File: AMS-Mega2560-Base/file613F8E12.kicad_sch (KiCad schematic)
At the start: 8 parts, among them IC18 MAX31865AAP+, J28 Conn_01x02, J29 Conn_01x03, J30 Conn_01x02

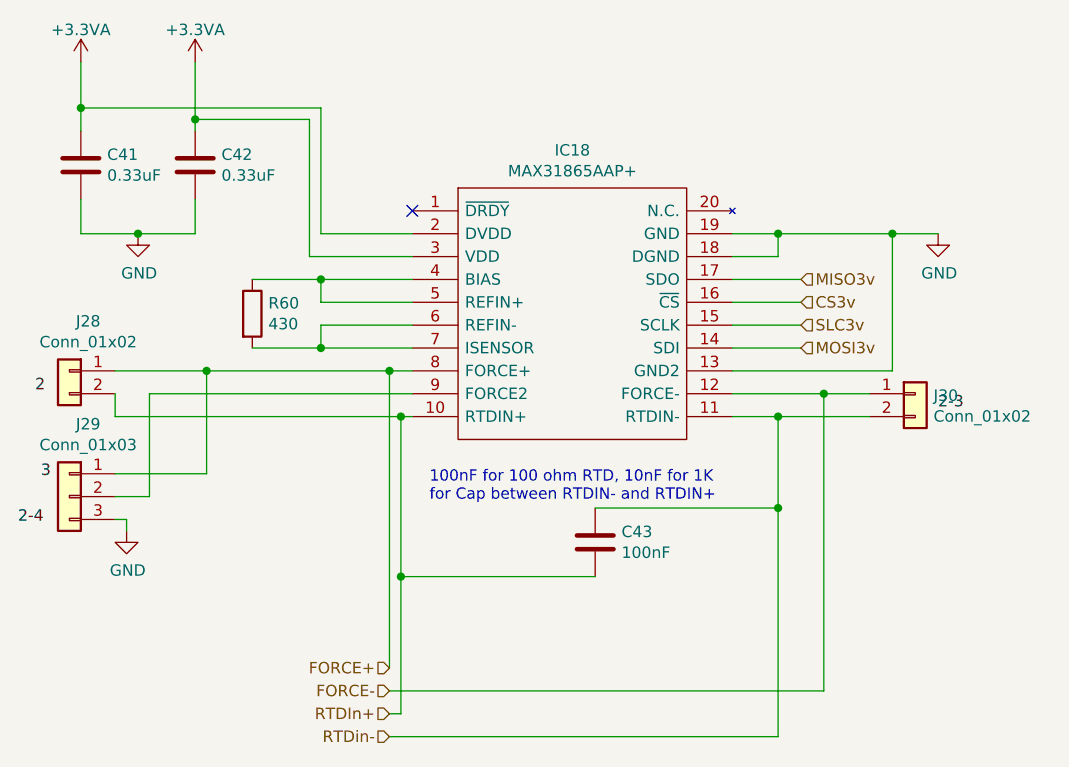
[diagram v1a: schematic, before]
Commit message: still fixing ERC stuff
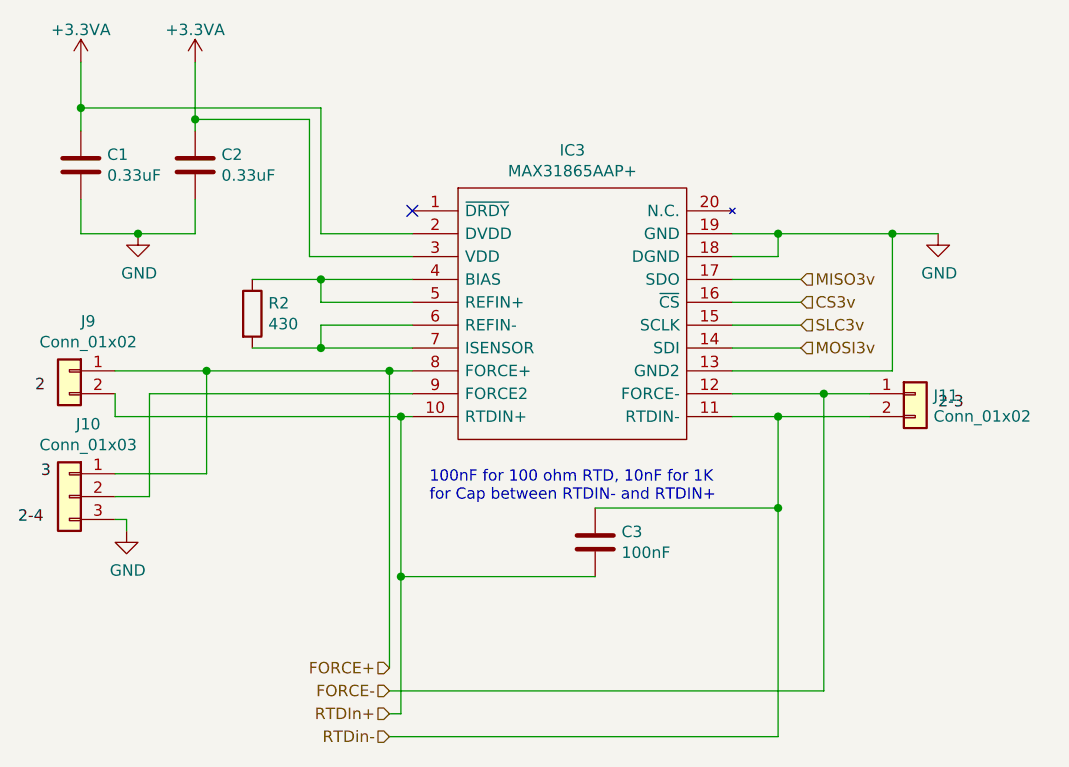
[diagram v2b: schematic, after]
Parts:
- renumbered C41 to C1, C42 to C2, C43 to C3, IC18 to IC3, J29 to J10, J30 to J11, J28 to J9, R60 to R2
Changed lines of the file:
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@@
   (symbol (lib_id "SamacSys_Parts:MAX31865AAP+") (at 135.89 77.47 0)
     (in_bom yes) (on_board yes)
-    (property "Reference" "IC18" (id 0) (at 153.67 70.739 0))
+    (property "Reference" "IC3" (id 0) (at 153.67 70.739 0))
     (property "Value" "MAX31865AAP+" (id 1) (at 153.67 73.0504 0))
     (property "Footprint" "SamacSys_Parts:SOP65P778X199-20N" (id 2) (at 167.64 74.93 0)
@@
   (symbol (lib_id "power:GND") (at 194.31 80.01 0)
     (in_bom yes) (on_board yes)
-    (property "Reference" "#PWR0124" (id 0) (at 194.31 86.36 0)
+    (property "Reference" "#PWR026" (id 0) (at 194.31 86.36 0)
       (effects (font (size 1.27 1.27)) hide)
     )
@@
   (symbol (lib_id "Device:C") (at 111.76 72.39 0)
     (in_bom yes) (on_board yes)
-    (property "Reference" "C42" (id 0) (at 114.681 71.2216 0)
+    (property "Reference" "C2" (id 0) (at 114.681 71.2216 0)
       (effects (font (size 1.27 1.27)) (justify left))
     )
@@
   (symbol (lib_id "Device:C") (at 99.06 72.39 0)
     (in_bom yes) (on_board yes)
-    (property "Reference" "C41" (id 0) (at 101.981 71.2216 0)
+    (property "Reference" "C1" (id 0) (at 101.981 71.2216 0)
       (effects (font (size 1.27 1.27)) (justify left))
     )
@@
   (symbol (lib_id "power:GND") (at 105.41 80.01 0)
     (in_bom yes) (on_board yes)
-    (property "Reference" "#PWR0122" (id 0) (at 105.41 86.36 0)
+    (property "Reference" "#PWR024" (id 0) (at 105.41 86.36 0)
       (effects (font (size 1.27 1.27)) hide)
     )
@@
   (symbol (lib_id "Device:R") (at 118.11 88.9 0)
     (in_bom yes) (on_board yes)
-    (property "Reference" "R60" (id 0) (at 119.888 87.7316 0)
+    (property "Reference" "R2" (id 0) (at 119.888 87.7316 0)
       (effects (font (size 1.27 1.27)) (justify left))
     )
@@
   (symbol (lib_id "power:GND") (at 104.14 113.03 0)
     (in_bom yes) (on_board yes)
-    (property "Reference" "#PWR0121" (id 0) (at 104.14 119.38 0)
+    (property "Reference" "#PWR023" (id 0) (at 104.14 119.38 0)
       (effects (font (size 1.27 1.27)) hide)
     )
@@
   (symbol (lib_id "Connector_Generic:Conn_01x02") (at 97.79 95.25 0) (mirror y)
     (in_bom yes) (on_board yes)
-    (property "Reference" "J28" (id 0) (at 99.8728 89.7382 0))
+    (property "Reference" "J9" (id 0) (at 99.8728 89.7382 0))
     (property "Value" "Conn_01x02" (id 1) (at 99.8728 92.0496 0))
     (property "Footprint" "Connector_PinHeader_2.54mm:PinHeader_1x02_P2.54mm_Vertical" (id 2) (at 97.79 95.25 0)
@@
   (symbol (lib_id "Connector_Generic:Conn_01x03") (at 97.79 109.22 0) (mirror y)
     (in_bom yes) (on_board yes)
-    (property "Reference" "J29" (id 0) (at 99.8728 101.1682 0))
+    (property "Reference" "J10" (id 0) (at 99.8728 101.1682 0))
     (property "Value" "Conn_01x03" (id 1) (at 99.8728 103.4796 0))
     (property "Footprint" "Connector_PinHeader_2.54mm:PinHeader_1x03_P2.54mm_Vertical" (id 2) (at 97.79 109.22 0)
@@
   (symbol (lib_id "Connector_Generic:Conn_01x02") (at 191.77 97.79 0)
     (in_bom yes) (on_board yes)
-    (property "Reference" "J30" (id 0) (at 193.802 97.9932 0)
+    (property "Reference" "J11" (id 0) (at 193.802 97.9932 0)
       (effects (font (size 1.27 1.27)) (justify left))
     )
@@
   (symbol (lib_id "Device:C") (at 156.21 114.3 0)
     (in_bom yes) (on_board yes)
-    (property "Reference" "C43" (id 0) (at 159.131 113.1316 0)
+    (property "Reference" "C3" (id 0) (at 159.131 113.1316 0)
       (effects (font (size 1.27 1.27)) (justify left))
     )
@@
   (symbol (lib_id "power:+3.3VA") (at 111.76 60.96 0)
     (in_bom yes) (on_board yes) (fields_autoplaced)
-    (property "Reference" "#PWR0134" (id 0) (at 111.76 64.77 0)
+    (property "Reference" "#PWR025" (id 0) (at 111.76 64.77 0)
       (effects (font (size 1.27 1.27)) hide)
     )
@@
   (symbol (lib_id "power:+3.3VA") (at 99.06 60.96 0)
     (in_bom yes) (on_board yes) (fields_autoplaced)
-    (property "Reference" "#PWR0130" (id 0) (at 99.06 64.77 0)
-      (effects (font (size 1.27 1.27)) hide)
-    )
+    (property "Reference" "#PWR022" (id 0) (at 99.06 64.77 0)
+      (effects (font (size 1.27 1.27)) hide)
+    )
